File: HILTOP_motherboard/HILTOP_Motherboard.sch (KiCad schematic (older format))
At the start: 209 parts, among them J1 BACKPLANE_PWR, J10 HDMI, J11 DISP_PWR, J12 DISPLAY_PORT, J14 VADJ_B, J15 VADJ_A, J16 SOFT_START_PWR, J17 PWR_LED, J18 USB_B, J19 Micro_SD_Card, J2 ATX_MOLEX_02X12, J20 CAMERA_PORT, J21 EXT_FAN, J22 BACKPLANE_LV_PWR, J23 EXT_FAN, J26 Conn_02x06_Odd_Even, J3 SATA, J4 USB_A_DOUBLE, J5 USB Front Panel, J6 Conn_02x05_Odd_Even, J7 Conn_02x08_Odd_Even, J8 EXT_TEMP_MON, J9 RJ45-TRANS_SI-61001-F, U1 LM337BD2TG, U25 STM6719SFWB6F, U39 MCP23017

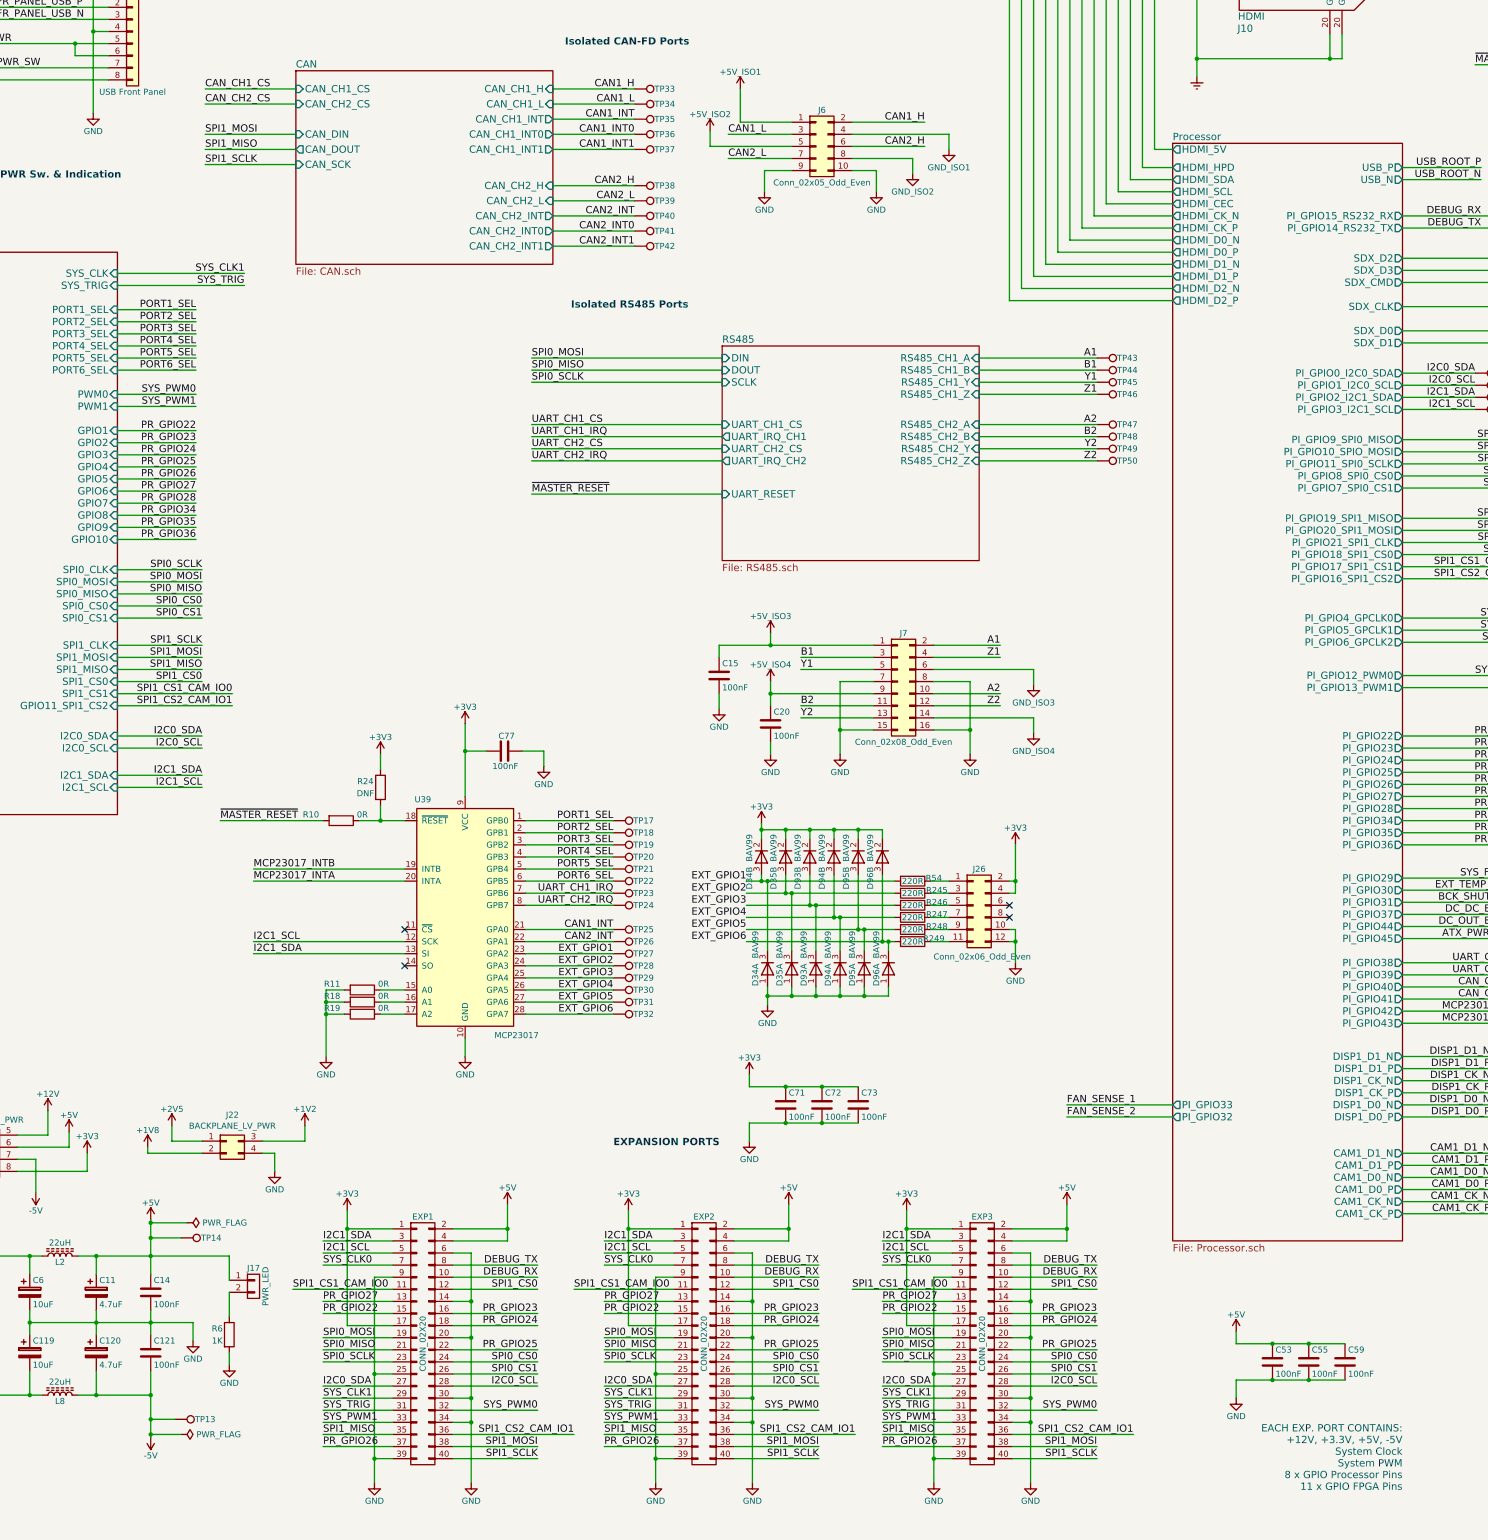
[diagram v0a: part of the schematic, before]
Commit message: nearly finished placing all parts!
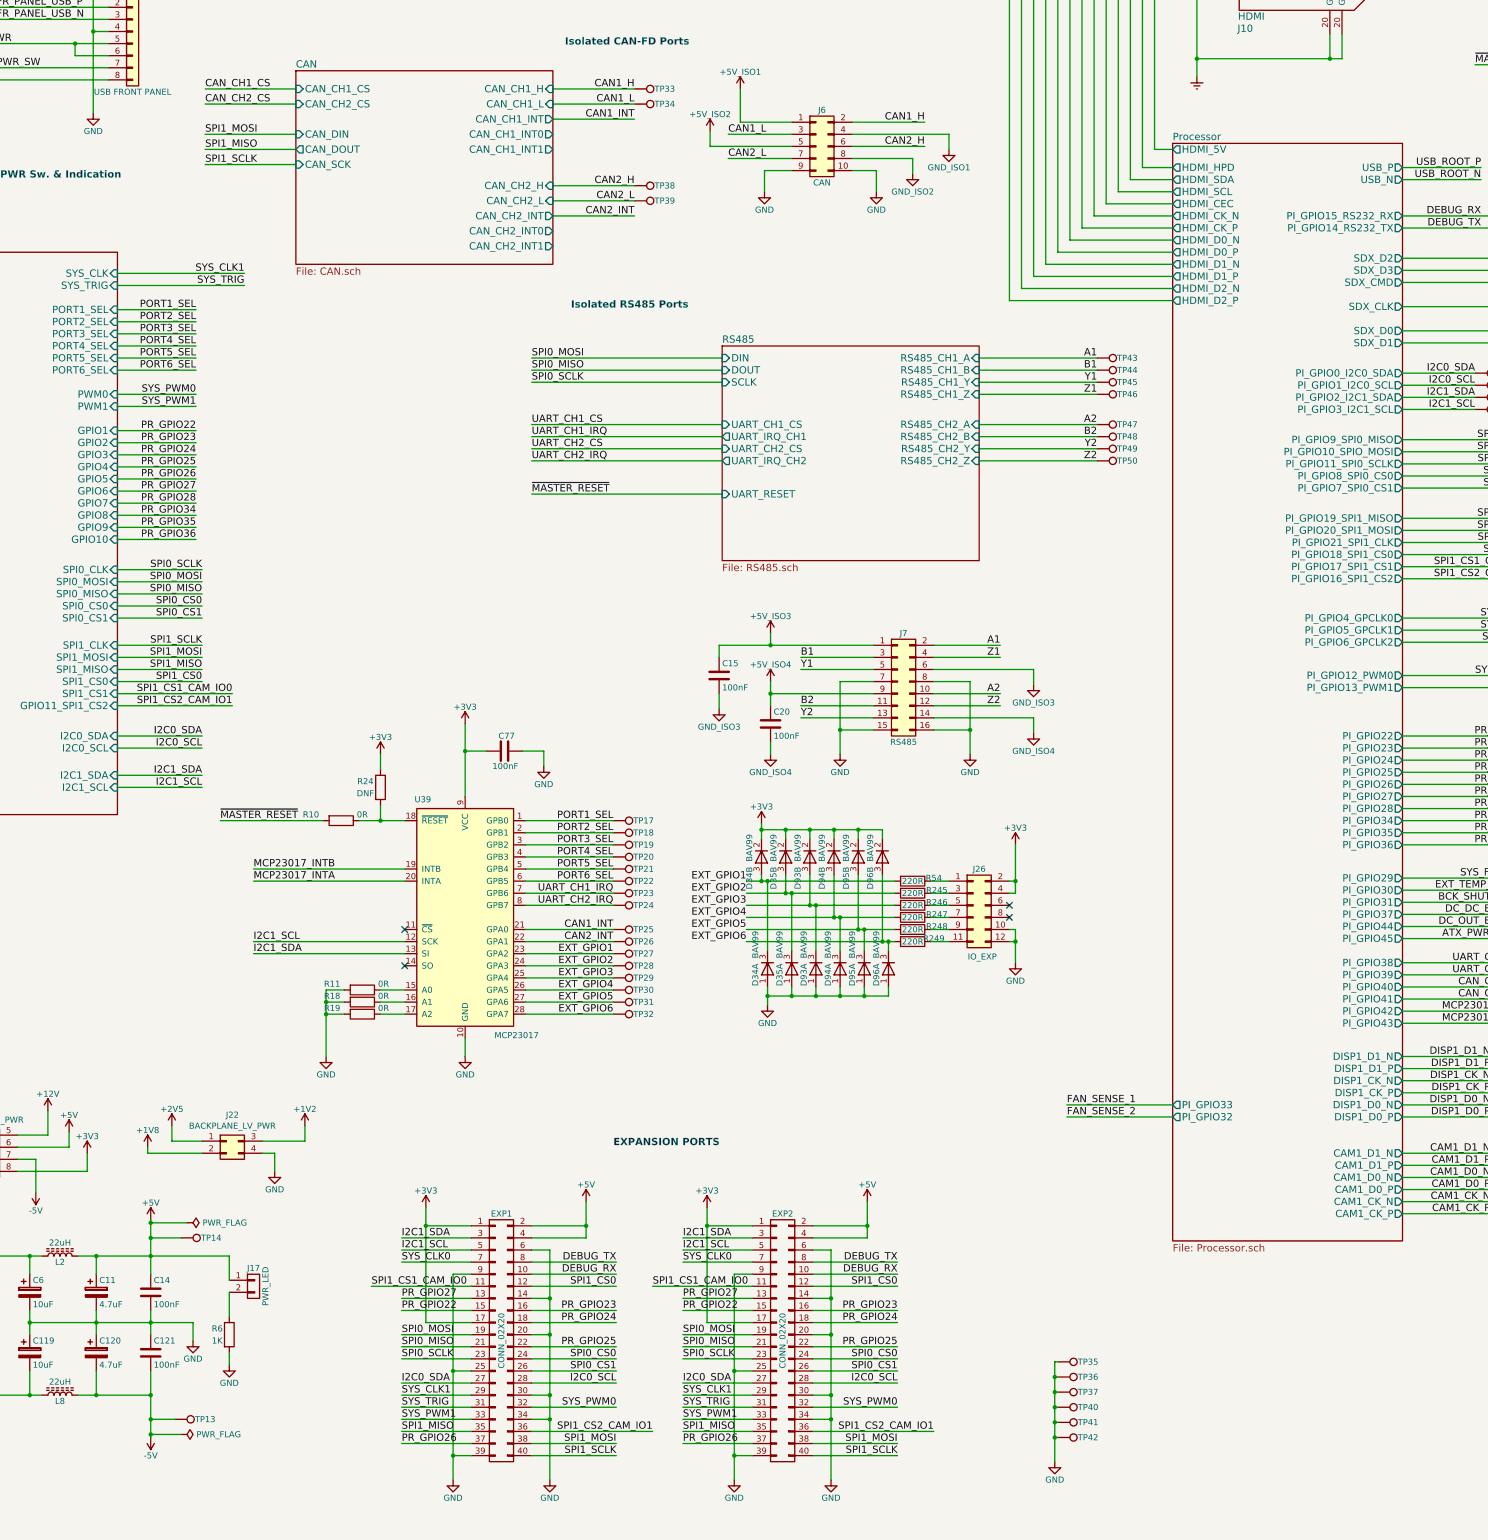
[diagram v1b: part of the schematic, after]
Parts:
- removed C53, C55: 100nF, Capacitor_SMD:C_0201_0603Metric, symbol device:C
- removed C59, C71, C72, C73: 100nF, Capacitor_SMD:C_0603_1608Metric, symbol device:C
- removed EXP3: CONN_02X20, Connector_IDC:IDC-Header_2x20_P2.54mm_Vertical, symbol HILTOP_Motherboard-rescue:CONN_02X20
- J1: Devtank (none) -> 709-005
- J18: Devtank (none) -> 703-002
- J21, J23: Devtank (none) -> 710-013
- J22: Devtank (none) -> 709-006
- J26: value Conn_02x06_Odd_Even -> IO_EXP; Devtank (none) -> 710-002
- J5: value USB Front Panel -> USB FRONT PANEL
- J6: value Conn_02x05_Odd_Even -> CAN; Devtank (none) -> 714-002
- J7: value Conn_02x08_Odd_Even -> RS485; Devtank (none) -> 714-004
- J8: Devtank (none) -> 710-014
- U39: footprint Package_SO:SOIC-28W_7.5x17.9mm_P1.27mm -> Package_SO:SSOP-28_5.3x10.2mm_P0.65mm
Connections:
- net CAN1_INT0 is gone; now on net GND: TP36.1
- net CAN1_INT1 is gone; now on net GND: TP37.1
- net CAN2_INT0 is gone; now on net GND: TP41.1
- net CAN2_INT1 is gone; now on net GND: TP42.1
- net CAN1_INT: no longer TP35.1
- net CAN2_INT: no longer TP40.1
- net GND: now also TP35.1, TP40.1; no longer C15.2, C20.2
- net GND_ISO3: now also C15.2
- net GND_ISO4: now also C20.2
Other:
- note removed: "EACH EXP. PORT CONTAINS:\n+12V, +3.3V, +5V, -5V\nSystem Clock\nSystem PWM\n8 x GPIO Processor Pins\n11 x GPIO FPGA Pins\n"
- moved on the sheet: EXP1, EXP2
